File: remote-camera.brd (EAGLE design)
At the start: 42.2 x 23.1 mm, 14 parts, among them Q1 IRF

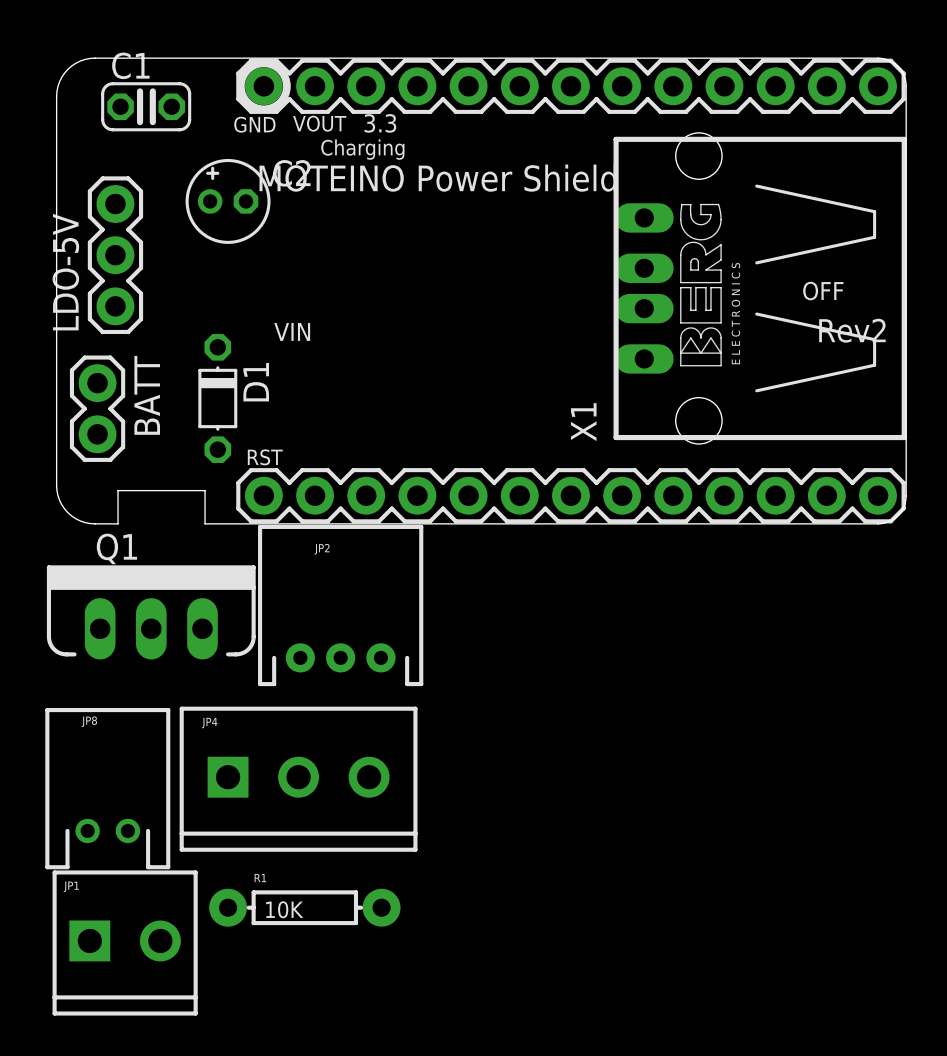
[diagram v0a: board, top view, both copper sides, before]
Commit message: update
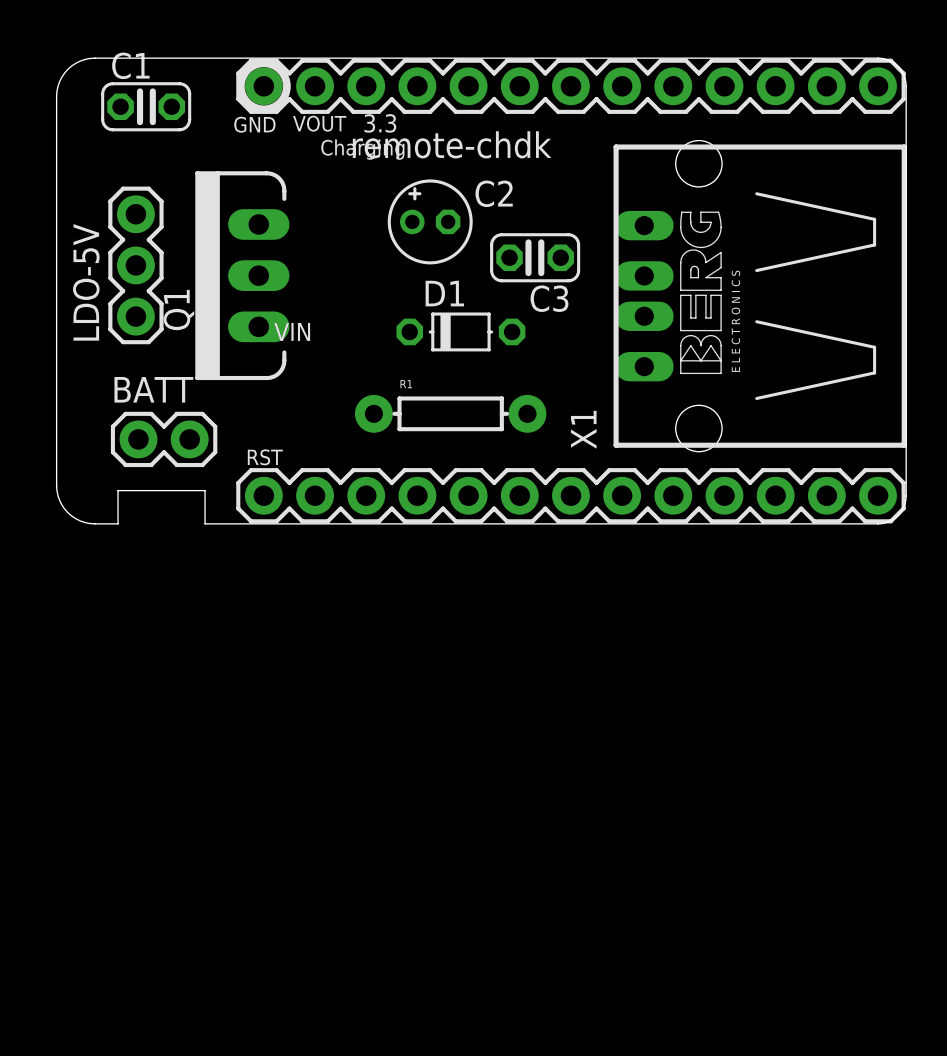
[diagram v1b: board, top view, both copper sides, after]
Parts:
- removed JP1: (no value), SparkFun:SCREWTERMINAL-3.5MM-2
- removed JP2: (no value), SparkFun:JST-3-PTH
- removed JP4: (no value), SparkFun:SCREWTERMINAL-3.5MM-3
- removed JP8: (no value), SparkFun:JST-2-PTH
- added C3: 0.1µ, resistor:C025-024X044
- moved R1 25.6 mm to (21.3, 5.46)
- moved Q1 18.3 mm to (11.8, 12.3), turned to 90 degrees
- moved D1 12.5 mm to (21.8, 9.53), turned to 0 degrees
- moved C2 10.1 mm to (20.3, 15.0)
- moved BATT 3.45 mm to (5.84, 4.19), turned to 0 degrees
- moved LDO-5V 1.14 mm to (5.71, 10.3)
- moved X1 0.38 mm to (33.7, 11.3)
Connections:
- removed net CONTROL: JP2.3, JP4.3, Q1.1, R1.P$2
- removed net HIGH-CURRENT: JP1.1, JP8.1, Q1.2
- new net N$2: C3.1, Q1.3
- net D3: now also Q1.1, R1.P$2
- net GND: now also C3.2, X1.4; no longer JP2.2, JP4.2, Q1.3
- net VCC: no longer JP1.2, JP2.1, JP4.1, JP8.2
- net VIN_MOTEINO: now also Q1.2, X1.1
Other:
- board text added: "remote-chdk"
- board text removed: "MOTEINO Power Shield"
- board text removed: "OFF"
- board text removed: "Rev2"
